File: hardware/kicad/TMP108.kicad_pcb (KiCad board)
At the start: 2 copper layers, 75 x 75 mm, 38 parts, among them J1 Screw_Terminal_01x08, J2 Screw_Terminal_01x08, J3 CAN, SW1 PRG, SW2 BUS, SW3 PRG-VALUE, U1 Teensy_3.2, U2 TMR-1211, U3 MCP2551-I-P

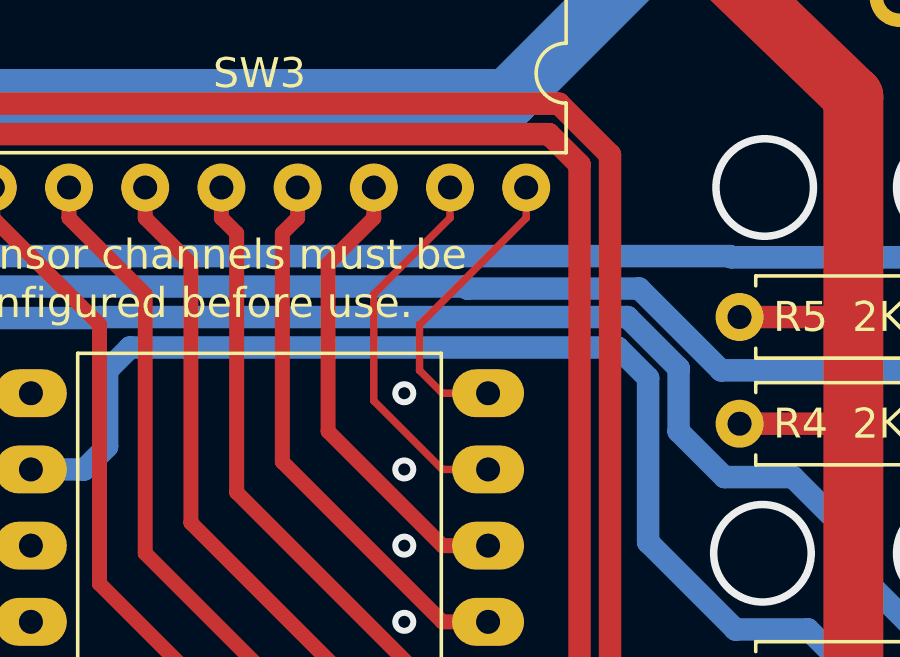
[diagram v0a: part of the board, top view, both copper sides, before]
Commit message: Tweaks
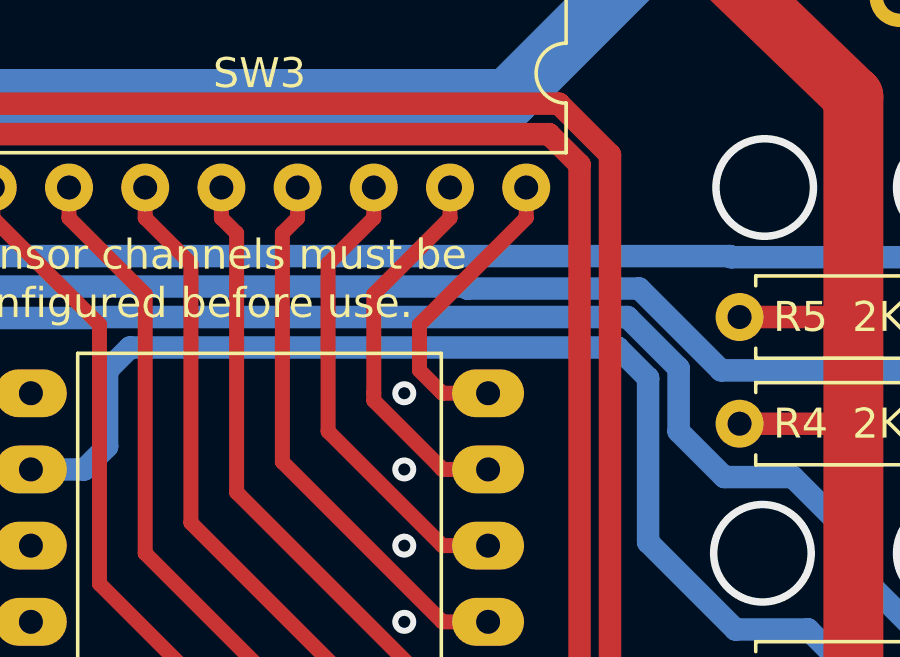
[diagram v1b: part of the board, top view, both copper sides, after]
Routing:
- net /ADDR_1: track 12.9 -> 16.4 mm
- net GND: vias 13 -> 19
- net (no net): vias 6 -> 0
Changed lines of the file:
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@@
     (thickness 1.6)
     (drawings 144)
-    (tracks 338)
+    (tracks 343)
     (zones 0)
     (modules 38)
@@
     (effects (font (size 1.5 1) (thickness 0.2)))
   )
-  (via (at 178.486 138.43) (size 0.8) (drill 0.4) (layers F.Cu B.Cu) (net 0))
-  (via (at 178.486 135.89) (size 0.8) (drill 0.4) (layers F.Cu B.Cu) (net 0))
-  (via (at 178.486 133.35) (size 0.8) (drill 0.4) (layers F.Cu B.Cu) (net 0))
-  (via (at 178.486 130.81) (size 0.8) (drill 0.4) (layers F.Cu B.Cu) (net 0))
-  (via (at 178.486 128.27) (size 0.8) (drill 0.4) (layers F.Cu B.Cu) (net 0))
-  (via (at 178.486 125.73) (size 0.8) (drill 0.4) (layers F.Cu B.Cu) (net 0))
+  (via (at 178.486 138.43) (size 0.8) (drill 0.4) (layers F.Cu B.Cu) (net 1))
+  (via (at 178.486 135.89) (size 0.8) (drill 0.4) (layers F.Cu B.Cu) (net 1))
+  (via (at 178.486 133.35) (size 0.8) (drill 0.4) (layers F.Cu B.Cu) (net 1))
+  (via (at 178.486 130.81) (size 0.8) (drill 0.4) (layers F.Cu B.Cu) (net 1))
+  (via (at 178.486 128.27) (size 0.8) (drill 0.4) (layers F.Cu B.Cu) (net 1))
+  (via (at 178.486 125.73) (size 0.8) (drill 0.4) (layers F.Cu B.Cu) (net 1))
   (via (at 178.486 123.19) (size 0.8) (drill 0.4) (layers F.Cu B.Cu) (net 1))
   (via (at 156.642 128.524) (size 3.5) (drill 3) (layers F.Cu B.Cu) (net 1))
@@
   (segment (start 177.47 117.348) (end 175.946 118.872) (width 0.5) (layer F.Cu) (net 24))
   (segment (start 177.47 116.332) (end 177.47 117.348) (width 0.5) (layer F.Cu) (net 24))
-  (segment (start 177.47 123.444) (end 179.756 125.73) (width 0.25) (layer F.Cu) (net 25))
-  (segment (start 177.47 119.888) (end 177.47 123.444) (width 0.25) (layer F.Cu) (net 25))
-  (segment (start 180.01 117.348) (end 177.47 119.888) (width 0.25) (layer F.Cu) (net 25))
-  (segment (start 180.01 116.332) (end 180.01 117.348) (width 0.25) (layer F.Cu) (net 25))
-  (segment (start 179.756 125.73) (end 181.28 125.73) (width 0.25) (layer F.Cu) (net 25))
-  (segment (start 182.55 116.332) (end 182.55 117.348) (width 0.25) (layer F.Cu) (net 26))
-  (segment (start 182.55 117.348) (end 178.994 120.904) (width 0.25) (layer F.Cu) (net 26))
-  (segment (start 178.994 120.904) (end 178.994 122.428) (width 0.25) (layer F.Cu) (net 26))
-  (segment (start 178.994 122.428) (end 179.756 123.19) (width 0.25) (layer F.Cu) (net 26))
-  (segment (start 179.756 123.19) (end 181.28 123.19) (width 0.25) (layer F.Cu) (net 26))
+  (segment (start 179.756 125.73) (end 179.629 125.603) (width 0.5) (layer F.Cu) (net 25))
+  (segment (start 181.28 125.73) (end 179.756 125.73) (width 0.5) (layer F.Cu) (net 25))
+  (segment (start 177.47 123.444) (end 179.629 125.603) (width 0.25) (layer F.Cu) (net 25))
+  (segment (start 179.756 125.718002) (end 177.47 123.432002) (width 0.5) (layer F.Cu) (net 25))
+  (segment (start 179.756 125.73) (end 179.756 125.718002) (width 0.5) (layer F.Cu) (net 25))
+  (segment (start 177.47 123.432002) (end 177.47 123.19) (width 0.5) (layer F.Cu) (net 25))
+  (segment (start 177.47 123.19) (end 177.47 123.444) (width 0.25) (layer F.Cu) (net 25))
+  (segment (start 177.47 123.19) (end 177.47 119.888) (width 0.5) (layer F.Cu) (net 25))
+  (segment (start 177.47 119.888) (end 180.01 117.348) (width 0.5) (layer F.Cu) (net 25))
+  (segment (start 180.01 117.348) (end 180.01 116.332) (width 0.5) (layer F.Cu) (net 25))
+  (segment (start 181.28 123.19) (end 179.756 123.19) (width 0.5) (layer F.Cu) (net 26))
+  (segment (start 179.756 123.19) (end 178.994 122.428) (width 0.5) (layer F.Cu) (net 26))
+  (segment (start 178.994 122.428) (end 178.994 120.904) (width 0.5) (layer F.Cu) (net 26))
+  (segment (start 178.994 120.904) (end 182.55 117.348) (width 0.5) (layer F.Cu) (net 26))
+  (segment (start 182.55 117.348) (end 182.55 116.332) (width 0.5) (layer F.Cu) (net 26))
   (segment (start 202.87 112.268) (end 202.87 102.616) (width 0.5) (layer B.Cu) (net 27))
   (segment (start 204.648 114.046) (end 202.87 112.268) (width 0.5) (layer B.Cu) (net 27))
@@
     (connect_pads (clearance 0.508))
     (min_thickness 0.254)
-    (fill (arc_segments 32) (thermal_gap 0.508) (thermal_bridge_width 0.508))
+    (fill yes (arc_segments 32) (thermal_gap 0.508) (thermal_bridge_width 0.508))
     (polygon
       (pts
@@
     (connect_pads (clearance 0.508))
     (min_thickness 0.254)
-    (fill (arc_segments 32) (thermal_gap 0.508) (thermal_bridge_width 0.508))
+    (fill yes (arc_segments 32) (thermal_gap 0.508) (thermal_bridge_width 0.508))
     (polygon
       (pts
